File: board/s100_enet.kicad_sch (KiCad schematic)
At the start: 34 parts, among them J1 FRAM socket, J2 SD Socket, J3 ClockSelect, P1 S100_MALE, SW1 SW_DIP_x08, U1 74LS10, U10 22V10, U11 74LS165, U12 74LS245, U13 74LS245, U14 74LS245, U15 74LS245, U2 74LS688, U3 74LS163, U4 74HC02, U5 L7805, U6 SPX2920U-3.3_TO220, U7 74LS138, U8 74LS595, U9 74LS175

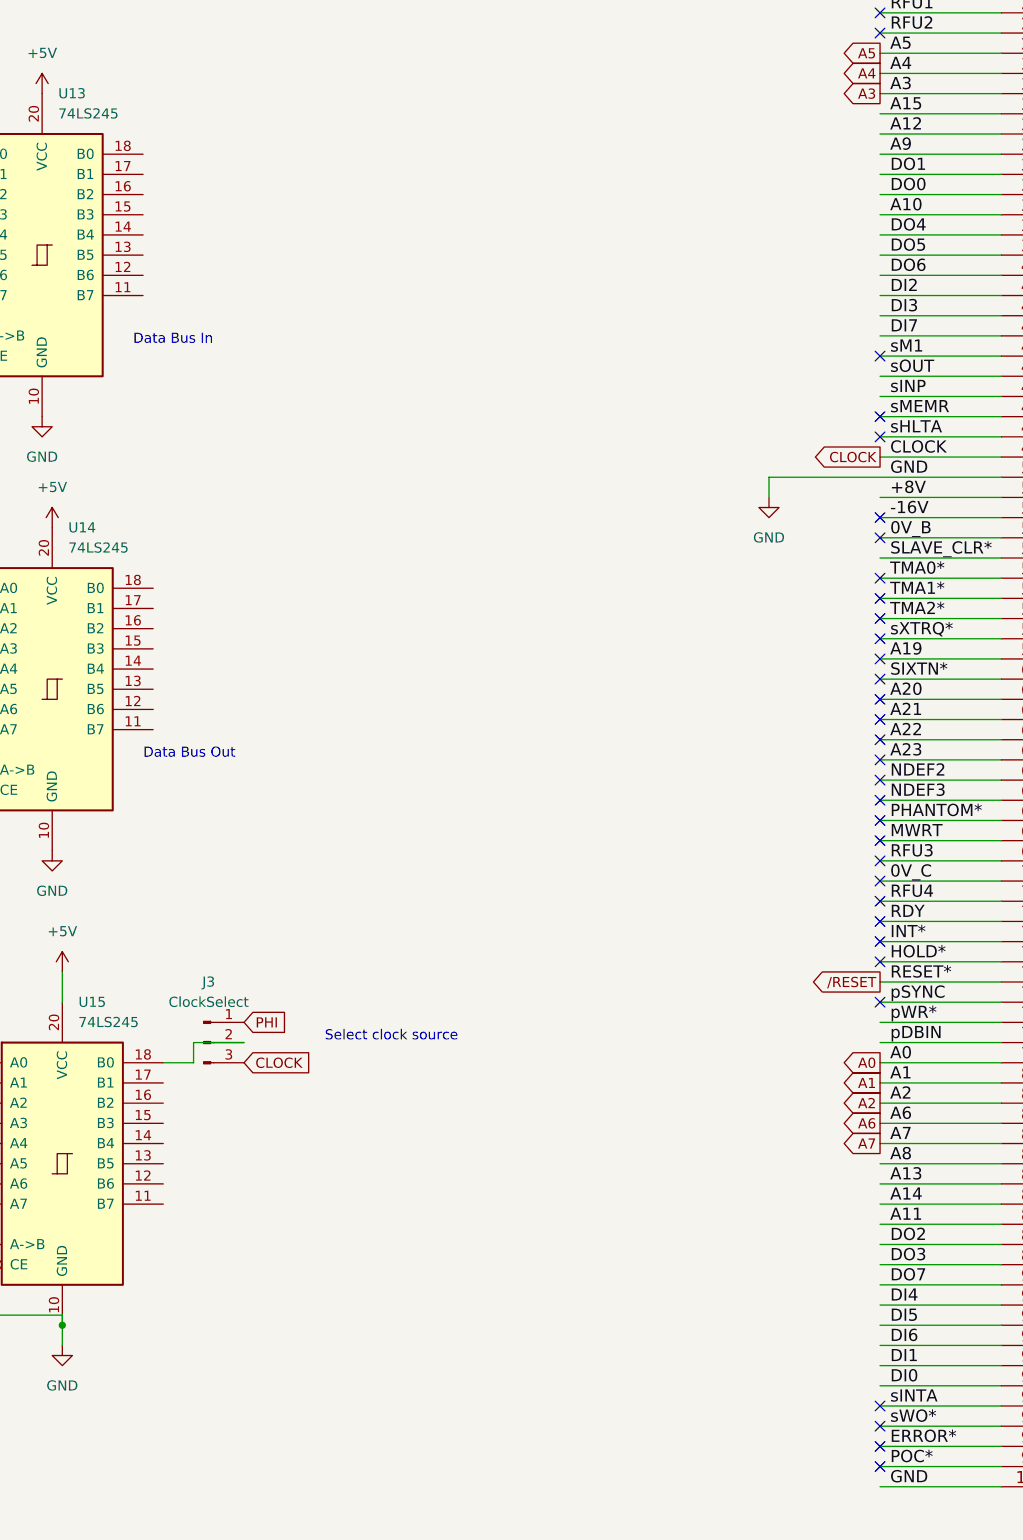
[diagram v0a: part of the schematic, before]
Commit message: update schmatic
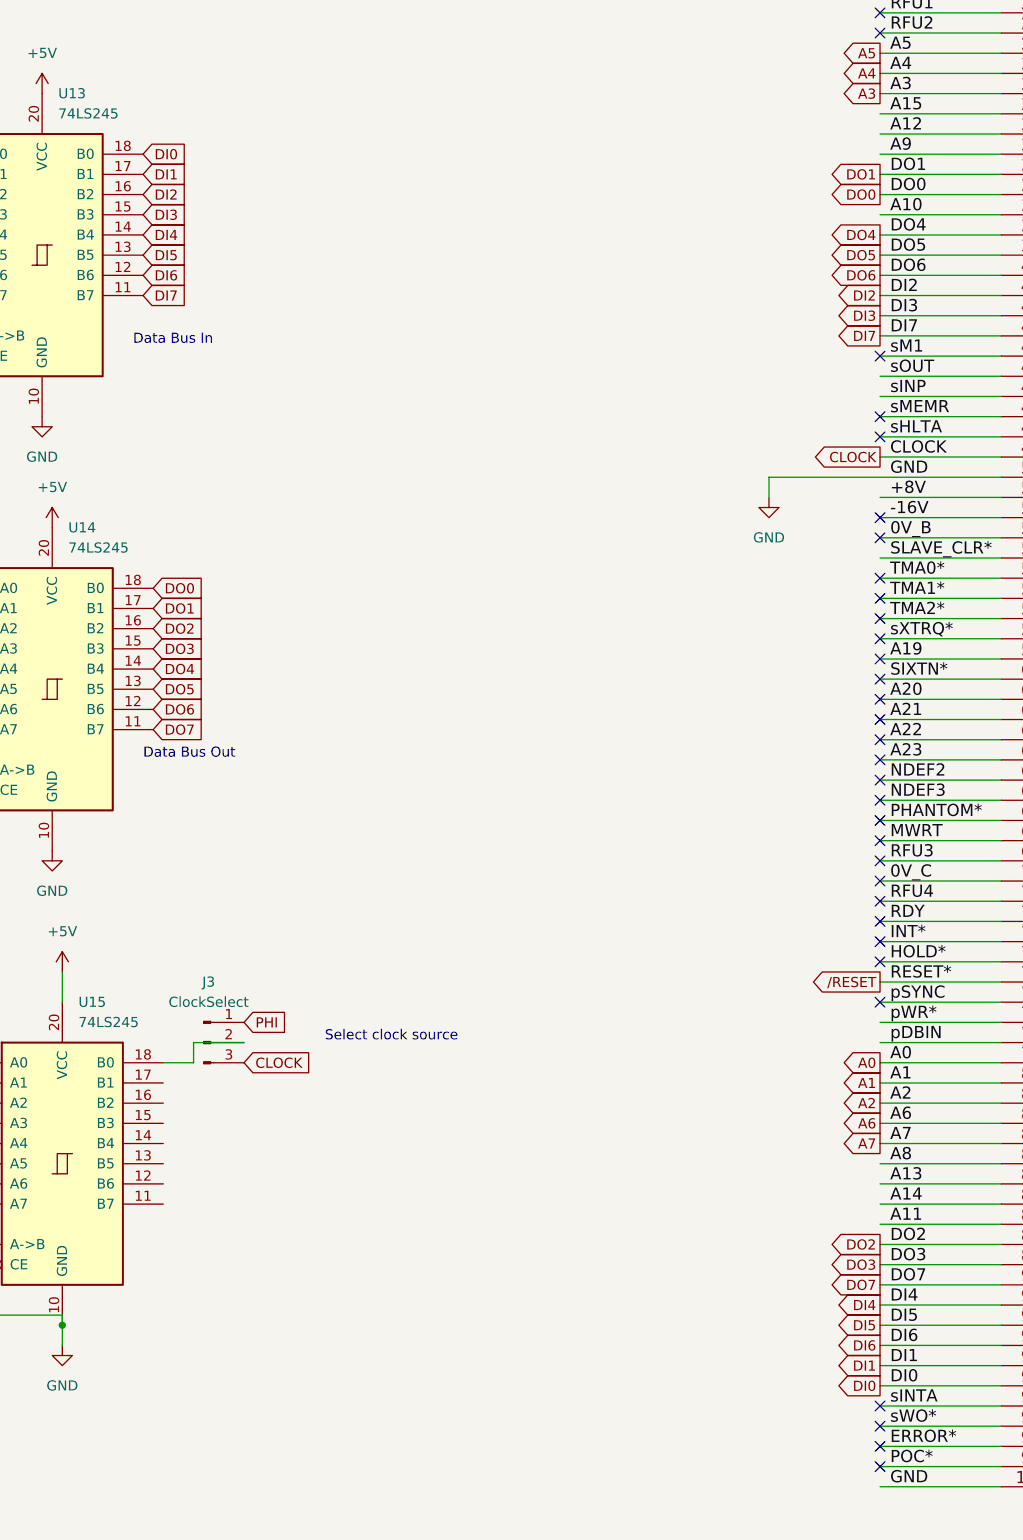
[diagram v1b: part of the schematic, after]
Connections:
- net DI0: now also U13.18 (B0)
- net DI1: now also U13.17 (B1)
- net DI2: now also U13.16 (B2)
- net DI3: now also U13.15 (B3)
- net DI4: now also U13.14 (B4)
- net DI5: now also U13.13 (B5)
- net DI6: now also U13.12 (B6)
- net DI7: now also U13.11 (B7)
- net DO0: now also U14.18 (B0)
- net DO1: now also U14.17 (B1)
- net DO2: now also U14.16 (B2)
- net DO3: now also U14.15 (B3)
- net DO4: now also U14.14 (B4)
- net DO5: now also U14.13 (B5)
- net DO6: now also U14.12 (B6)
- net DO7: now also U14.11 (B7)
